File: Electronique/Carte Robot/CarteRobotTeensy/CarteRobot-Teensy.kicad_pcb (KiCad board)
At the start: 2 copper layers, 95.5 x 88.5 mm, 52 parts, among them J1 Conn_Bat2, J10 Conn_01x03, J11 Conn_01x05, J12 Conn_01x05, J13 Conn_01x04, J14 Conn_02x04_Counter_Clockwise, J15 Shield-Actionneurs, J16 Conn_Aru, J17 Conn_Aru, J18 Conn_Aru, J19 Conn_IHM, J2 Conn_Bat1, J20 Conn_Aru, J21 Conn_Aru, J22 Conn_01x03, J3 Conn_OnOff, J4 Conn_Aru, J5 Teensy-3.5, J6 Conn_DriverD, J7 Conn_DriverG, J8 Conn_01x03, J9 Conn_01x03, U1 TSR_1-2450

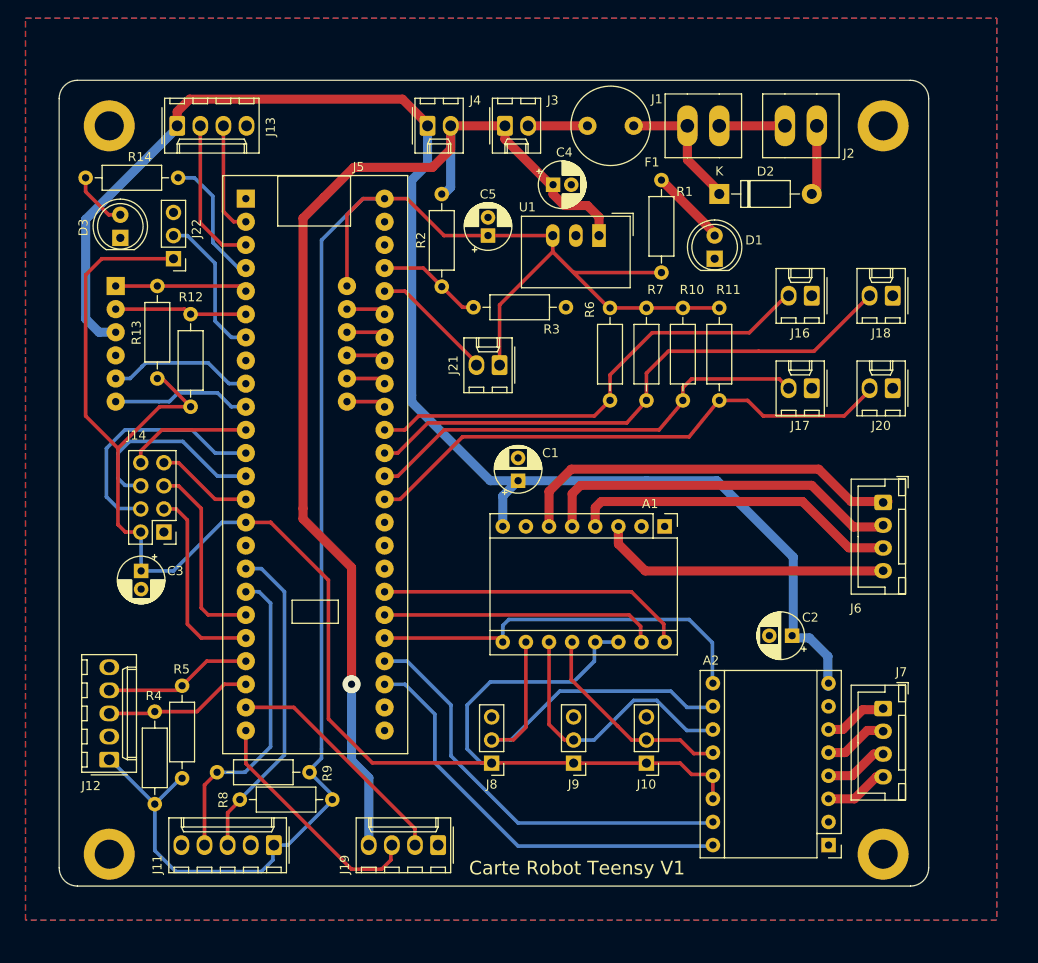
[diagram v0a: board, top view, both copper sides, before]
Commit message: gerbers
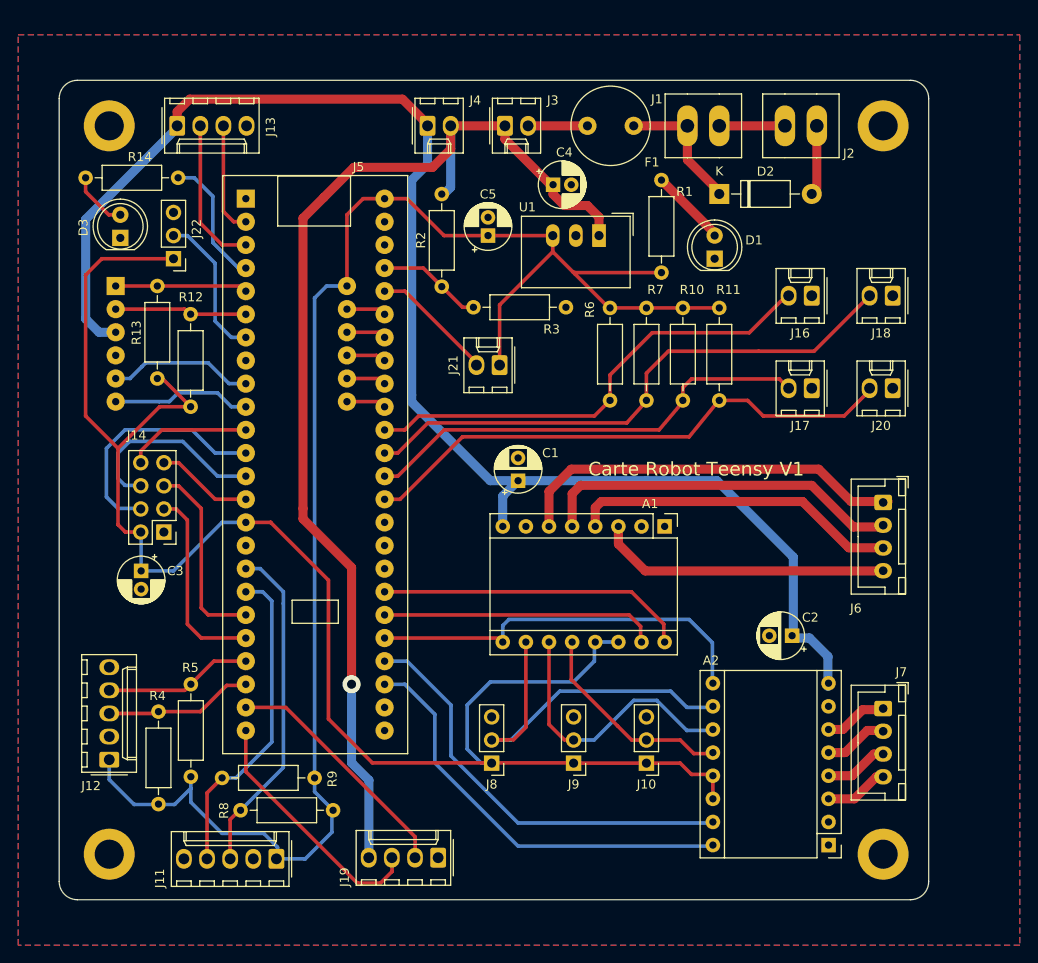
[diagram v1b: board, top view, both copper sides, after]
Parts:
- moved J11 1.53 mm to (78.4, 135.5)
- moved J19 1.38 mm to (96.1, 135.4)
- moved R8 1.18 mm to (84.6, 130.2)
- moved R5 0.98 mm to (69.0, 126.5)
- moved R9 0.83 mm to (82.5, 126.6)
- moved R4 0.41 mm to (65.4, 129.5)
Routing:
- net +5V: track 194.8 -> 181.7 mm
- net /CODG_A: track 36.0 -> 37.7 mm
- net /Von: track 126.3 -> 127.8 mm
- net /RX4: track 26.0 -> 27.3 mm
- net /CODD_B: track 16.0 -> 17.1 mm
- net /CODG_B: track 34.7 -> 35.8 mm
- net /TX4: track 26.8 -> 27.7 mm
- net /CODD_A: track 17.1 -> 16.3 mm
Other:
- board size 95.5 x 88.5 mm -> 95.5 x 90 mm
